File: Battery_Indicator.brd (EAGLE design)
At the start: 41.9 x 29.5 mm, 33 parts, among them IC1 MEGA8-AI, IC2 7805DT, Q1 IRF3704S, Q2 IRF3704S

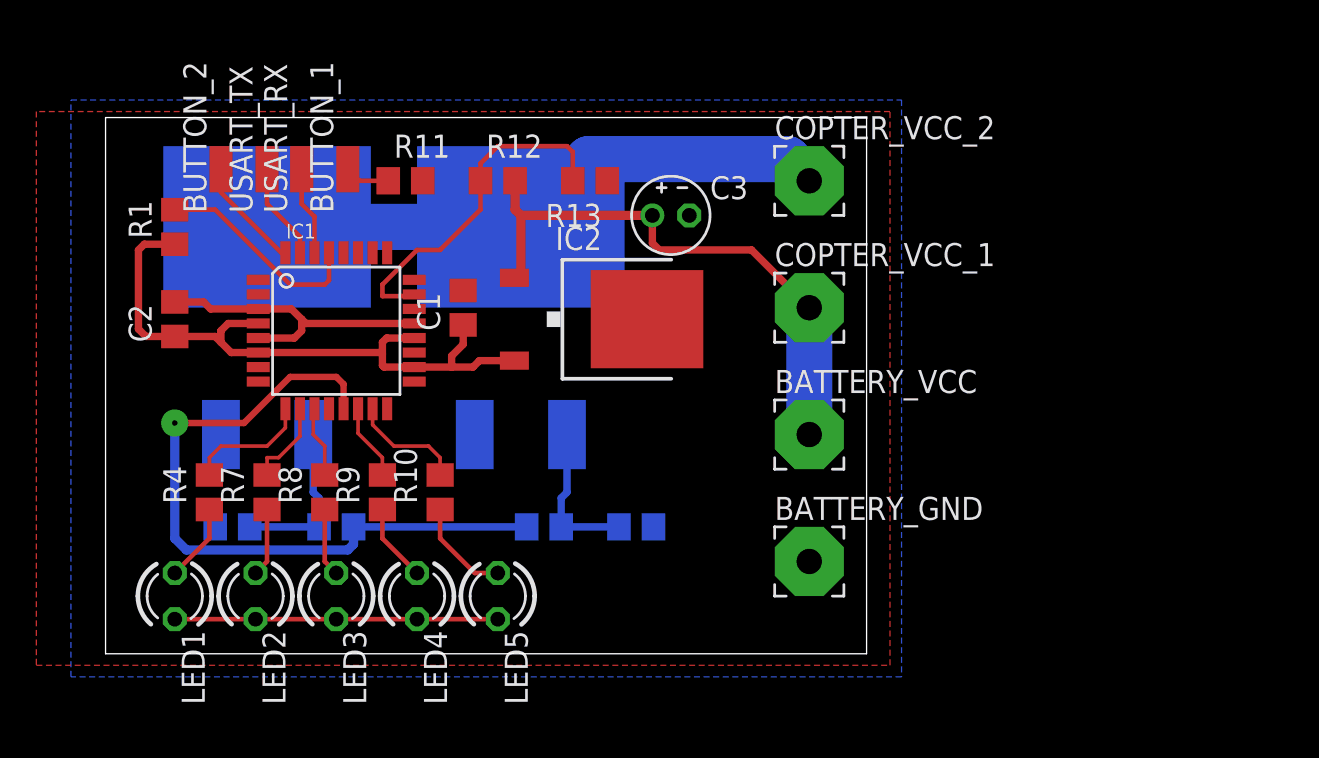
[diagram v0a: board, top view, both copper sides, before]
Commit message: Update EAGLE project files
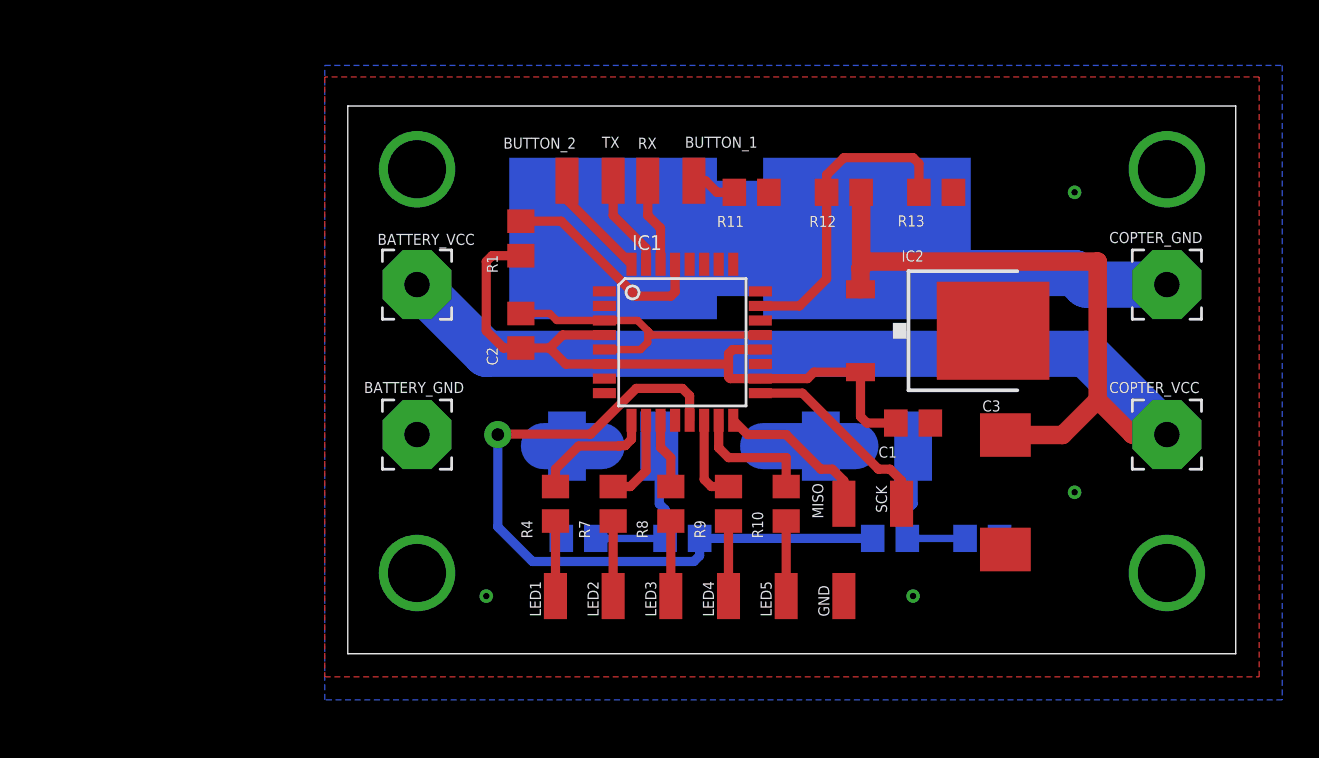
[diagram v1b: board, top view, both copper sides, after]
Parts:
- removed COPTER_VCC_1, COPTER_VCC_2: (no value), wirepad:3,81/1,4
- removed USART_RX, USART_TX: (no value), wirepad:SMD1,27-2,54
- added COPTER_GND, COPTER_VCC: (no value), wirepad:3,81/1,4
- added GND, MISO, RX, SCK, TX: (no value), wirepad:SMD1,27-2,54
- C3: device rcl:E2-4 -> rcl:SMC_D
- IC1: value MEGA8-AI -> ATMEGA8
- LED1: value RED 1st -> (none); device led:LED3MM -> wirepad:SMD1,27-2,54
- LED2: value GREEN 2nd -> (none); device led:LED3MM -> wirepad:SMD1,27-2,54
- LED3: value GREEN 3rd -> (none); device led:LED3MM -> wirepad:SMD1,27-2,54
- LED4: value GREEN 4th -> (none); device led:LED3MM -> wirepad:SMD1,27-2,54
- LED5: value GREEN 5th -> (none); device led:LED3MM -> wirepad:SMD1,27-2,54
- moved C1 25.6 mm to (44.5, 88.9), turned to 0 degrees
- moved C3 23.9 mm to (49.5, 85.1), turned to 270 degrees
- moved BATTERY_VCC 23.1 mm to (17.1, 96.5), turned to 90 degrees
- moved BATTERY_GND 22.7 mm to (17.1, 88.3)
- moved LED1 21.0 mm to (24.8, 79.4), turned to 0 degrees
- moved LED2 19.7 mm to (27.9, 79.4), turned to 0 degrees
- moved R10 19.1 mm to (37.5, 84.5)
- moved C2 19.1 mm to (22.9, 94.0)
- moved IC1 19.1 mm to (31.8, 93.3)
- moved Q1 19.1 mm to (27.9, 96.5)
- moved R1 19.1 mm to (22.9, 99.1)
- moved R11 19.1 mm to (35.6, 101.6)
- moved R12 19.1 mm to (40.6, 101.6)
- moved R2 19.1 mm to (31.8, 82.5)
- moved R3 19.1 mm to (43.2, 82.5)
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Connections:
- new net N$25: IC1.16, MISO.1
- new net N$26: IC1.17, SCK.1
- net +24V: now also COPTER_VCC.1; no longer COPTER_VCC_1.1
- net GND: now also GND.1; no longer LED1.K, LED2.K, LED3.K, LED4.K, LED5.K
- net N$10: now also LED4.1; no longer LED4.A
- net N$11: now also LED5.1; no longer LED5.A
- net N$17: now also RX.1; no longer USART_RX.1
- net N$20: now also TX.1; no longer USART_TX.1
- net N$5: now also COPTER_GND.1; no longer COPTER_VCC_2.1
- net N$7: now also LED1.1; no longer LED1.A
- net N$8: now also LED2.1; no longer LED2.A
- net N$9: now also LED3.1; no longer LED3.A
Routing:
- net +24V: track 31.5 -> 81.3 mm
- net N$5: track 35.0 -> 65.4 mm
- net N$26: track 0.00 -> 11.0 mm
- net GND: track 34.6 -> 25.1 mm, vias 0 -> 4
- net N$25: track 0.00 -> 8.74 mm
- net N$19: track 19.3 -> 17.2 mm
- net N$6: track 38.9 -> 40.7 mm
- net +5V: track 36.9 -> 38.4 mm
- net N$11: track 5.55 -> 4.13 mm
- net N$16: track 6.30 -> 7.05 mm
- net N$15: track 4.20 -> 4.76 mm
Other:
- board size 41.9 x 29.5 mm -> 48.9 x 30.1 mm
